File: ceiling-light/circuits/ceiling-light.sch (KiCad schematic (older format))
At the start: 33 parts, among them J1 Screw_Terminal_01x03, J2 Screw_Terminal_01x02, J3 Conn_02x04_Counter_Clockwise, Q2 IRF840, Q3 IRF840, Q4 KSP44, SW1 SW_Push, SW2 SW_Push, U1 LTV-817, U2 HLK-PM05, U3 AMS1117-3.3, U4 FL51xxMX, U5 TMP36xS, U6 ESP32-WROOM-32D

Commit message: removed old undimmable version
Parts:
- BR1: symbol ceiling-light-dimmable-rescue:DB107-BP-Diode_Bridge_slimc-ceiling-light-dimmable-rescue-ceiling-light-dimmable-rescue -> ceiling-light-rescue:DB107-BP-Diode_Bridge_slimc-ceiling-light-dimmable-rescue-ceiling-light-dimmable-rescue-ceiling-li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
- U4: symbol ceiling-light-dimmable-rescue:FL51xxMX-AC_Drivers_slimc-ceiling-light-dimmable-rescue-ceiling-light-dimmable-rescue -> ceiling-light-rescue:FL51xxMX-AC_Drivers_slimc-ceiling-light-dimmable-rescue-ceiling-light-dimmable-rescue-ceiling-ligh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
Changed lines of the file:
@@
 EESchema Schematic File Version 4
-LIBS:ceiling-light-dimmable-cache
+LIBS:ceiling-light-cache
 EELAYER 26 0
 EELAYER END
@@
 	6400 700  6400 4400
 $Comp
-L ceiling-light-dimmable-rescue:FL51xxMX-AC_Drivers_slimc-ceiling-light-dimmable-rescue-ceiling-light-dimmable-rescue U4
+L ceiling-light-rescue:FL51xxMX-AC_Drivers_slimc-ceiling-light-dimmable-rescue-ceiling-light-dimmable-rescue-ceiling-light-dimmable-rescue-ceiling-light-dimmable-rescue U4
 U 1 1 5D445EC1
 P 4600 1500
@@
 $EndComp
 $Comp
-L ceiling-light-dimmable-rescue:DB107-BP-Diode_Bridge_slimc-ceiling-light-dimmable-rescue-ceiling-light-dimmable-rescue BR1
+L ceiling-light-rescue:DB107-BP-Diode_Bridge_slimc-ceiling-light-dimmable-rescue-ceiling-light-dimmable-rescue-ceiling-light-dimmable-rescue-ceiling-light-dimmable-rescue BR1
 U 1 1 5D4584FE
 P 4400 3450

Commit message: new schematic layout
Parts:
- removed BR1: DB107-BP, Diode_THT_slimc:DB107-BP, symbol ceiling-light-rescue:DB107-BP-Diode_Bridge_slimc-ceiling-light-dimmable-rescue-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
- removed J3: Conn_02x04_Counter_Clockwise, Connector_PinSocket_2.54mm:PinSocket_2x04_P2.54mm_Vertical, symbol Connector_Generic:Conn_02x04_Counter_Clockwise
- removed R7: LDR03, OptoDevice:R_LDR_5.0x4.1mm_P3mm_Vertical, symbol Sensor_Optical:LDR03
- removed SW2: SW_Push, Button_Switch_THT:SW_Tactile_Straight_KSA0Axx1LFTR, symbol Switch:SW_Push
- removed U4: FL51xxMX, AC_Drivers_slimc:FL51xxMX, symbol ceiling-light-rescue:FL51xxMX-AC_Drivers_slimc-ceiling-light-dimmable-rescue-ce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
- added BR1: DB107-BP, DIP825W56P510L828H330Q4N, symbol Diode_Bridge_slimc:DB107-BP
- added J3: Conn_01x04, symbol Connector_Generic:Conn_01x04
- added R3: LDR03, OptoDevice:R_LDR_5.0x4.1mm_P3mm_Vertical, symbol Sensor_Optical:LDR03
- added R4: 6K8, Resistor_THT:R_Axial_DIN0207_L6.3mm_D2.5mm_P10.16mm_Horizontal, symbol Device:R
- added U4: FL51xxMX, symbol AC_Drivers_slimc:FL51xxMX
- C1, C4: value 100nF -> 100n
- C2: value 22nF -> 22n
- R6: value 6K8 -> 10K
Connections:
- net labels removed: +5V, ESP_EN, ESP_GPIO_00, ESP_GPIO_02, ESP_GPIO_04, ESP_GPIO_05, ESP_GPIO_12, ESP_GPIO_13, ESP_GPIO_14, ESP_GPIO_15, ESP_GPIO_16, ESP_GPIO_17, ESP_GPIO_18, ESP_GPIO_19, ESP_GPIO_21, ESP_GPIO_22, ESP_GPIO_23, ESP_GPIO_25, ESP_GPIO_26, ESP_GPIO_27, ESP_GPIO_33, ESP_GPIO_34, ESP_GPIO_35, ESP_RXD0, ESP_SENSOR_VN, ESP_SENSOR_VP, ESP_TXD0, L_M1, L_M2, L_OUT, N_MAIN
- wire segments 151 -> 157
- no-connect marks 22 -> 25
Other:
- note added: "AC LOAD OUTPUT"
- note added: "AC SENSE (ZERO CROSSING)"
- note added: "FTDI"
- note added: "LAMP SOCKET INPUT"
- note added: "LIGHT LEVEL SENSE"
- note added: "LOAD CONTROL (DIMMABLE)"
- note added: "MCU (ESP32)"
- note added: "PCB TEMP MONITOR"
- note added: "POWER SUPPLY"
- note removed: "3V3 DC CONVERTER"
- note removed: "5 : GND"
- note removed: "5V ACDC CONVERTER"
- note removed: "6 : GND"
- note removed: "7 : 5V PWR"
- note removed: "8 : 3V3 PWR"
- note removed: "ESP32-WROOM-32D MCU"
- note removed: "FTDI DTR -> ESP GPIO0 : 4"
- note removed: "FTDI RTS -> ESP EN : 3"
- note removed: "FTDI RXD -> ESP TXD : 1"
- note removed: "FTDI TXD -> ESP RXD : 2"
- note removed: "LIGHT SENSER"
- note removed: "MAINS INPUT"
- note removed: "MAINS OUTPUT"
- note removed: "MAINS POWER SENSE"
- note removed: "MAINS POWER SWITCHING"
- note removed: "PROGRAMMING HEADER"
- note removed: "TEMPERATURE SENSOR"
- moved on the sheet: C1, C2, C3, C4, D2, F1, J1, J2, Q2, Q3, Q4, R1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

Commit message: work on dimmable ceiling light
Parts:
- removed C1, C4: 100n, Capacitor_THT:CP_Radial_D5.0mm_P2.50mm, symbol Device:C_Small
- removed J3: Conn_01x04, symbol Connector_Generic:Conn_01x04
- removed U3: AMS1117-3.3, Package_TO_SOT_SMD:SOT-223-3_TabPin2, symbol Regulator_Linear:AMS1117-3.3
- added C1, C4: 0.1µ, Capacitor_THT:CP_Radial_D5.0mm_P2.50mm, symbol Device:CP
- added J3: Conn_01x06, symbol Connector_Generic:Conn_01x06
- added R7: 10K, Resistor_THT:R_Axial_DIN0207_L6.3mm_D2.5mm_P10.16mm_Horizontal, symbol Device:R
- added SW2: SW_Push, Button_Switch_THT:SW_Tactile_Straight_KSA0Axx1LFTR, symbol Switch:SW_Push
- BR1: value DB107-BP -> DB107; footprint DIP825W56P510L828H330Q4N -> (none)
- U2: value HLK-PM05 -> HLK-PM03
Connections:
- wire segments 157 -> 165
- no-connect marks 25 -> 24
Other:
- note added: "FTDI HEADER"
- note removed: "FTDI"
- moved on the sheet: C2, C3, C5, D1, D2, F1, J1, J2, Q2, Q3, Q4, R1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

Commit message: changed schematic layout
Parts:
- removed BR1: DB107, symbol Diode_Bridge_slimc:DB107-BP
- removed C1, C4, C5: 0.1µ, Capacitor_THT:CP_Radial_D5.0mm_P2.50mm, symbol Device:CP
- removed C2: 22n, Capacitor_THT:CP_Radial_D5.0mm_P2.50mm, symbol Device:C_Small
- removed C3: 4µ7, Capacitor_THT:CP_Radial_D5.0mm_P2.50mm, symbol Device:CP
- removed D1: WS2812B, LED_SMD:LED_WS2812B_PLCC4_5.0x5.0mm_P3.2mm, symbol LED:WS2812B
- removed D2: 1N4007, Diode_THT:D_DO-41_SOD81_P10.16mm_Horizontal, symbol Diode:1N4007
- removed F1: Fuse, Fuse_Holders_and_Fuses:Fuseholder5x20_horiz_open_lateral_Type-II, symbol Device:Fuse
- removed J1: Screw_Terminal_01x03, TerminalBlock:TerminalBlock_bornier-3_P5.08mm, symbol Connector:Screw_Terminal_01x03
- removed J2: Screw_Terminal_01x02, TerminalBlock:TerminalBlock_bornier-2_P5.08mm, symbol Connector:Screw_Terminal_01x02
- removed J3: Conn_01x06, symbol Connector_Generic:Conn_01x06
- removed Q2, Q3: IRF840, Package_TO_SOT_SMD:TO-263-3_TabPin2, symbol Transistor_FET:IRF740
- removed Q4: KSP44, Package_TO_SOT_THT:TO-92_Inline, symbol Transistor_BJT:2N2219
- removed R1: 390K, Resistor_THT:R_Axial_DIN0207_L6.3mm_D2.5mm_P10.16mm_Horizontal, symbol Device:R
- removed R10, R12, R13: 2M2, Resistor_THT:R_Axial_DIN0411_L9.9mm_D3.6mm_P12.70mm_Horizontal, symbol Device:R
- removed R11: 1K, Resistor_THT:R_Axial_DIN0207_L6.3mm_D2.5mm_P10.16mm_Horizontal, symbol Device:R
- removed R2, R6, R7: 10K, Resistor_THT:R_Axial_DIN0207_L6.3mm_D2.5mm_P10.16mm_Horizontal, symbol Device:R
- removed R3: LDR03, OptoDevice:R_LDR_5.0x4.1mm_P3mm_Vertical, symbol Sensor_Optical:LDR03
- removed R4: 6K8, Resistor_THT:R_Axial_DIN0207_L6.3mm_D2.5mm_P10.16mm_Horizontal, symbol Device:R
- removed R5: 330K, Resistor_THT:R_Axial_DIN0207_L6.3mm_D2.5mm_P10.16mm_Horizontal, symbol Device:R
- removed R9: 33K, Resistor_THT:R_Axial_DIN0207_L6.3mm_D2.5mm_P10.16mm_Horizontal, symbol Device:R
- removed SW1, SW2: SW_Push, Button_Switch_THT:SW_Tactile_Straight_KSA0Axx1LFTR, symbol Switch:SW_Push
- removed U1: LTV-817, Package_DIP:DIP-4_W7.62mm, symbol Isolator:LTV-817
- removed U2: HLK-PM03, Power_Supply:HLK-PM01, symbol Power_Supplies:HLK-PM05
- removed U4: FL51xxMX, symbol AC_Drivers_slimc:FL51xxMX
- removed U5: TMP36xS, Package_SO:SOIC-8_3.9x4.9mm_P1.27mm, symbol Sensor_Temperature:TMP36xS
- removed U6: ESP32-WROOM-32D, RF_Module:ESP32-WROOM-32, symbol RF_Module:ESP32-WROOM-32D
- added C? (x2): 0.1µ, Capacitor_THT:CP_Radial_D5.0mm_P2.50mm, symbol Device:CP
- added C?: 22n, Capacitor_THT:CP_Radial_D5.0mm_P2.50mm, symbol Device:C_Small
- added C? (x2): 0.1µ, symbol Device:CP_Small
- added C?: 22µ, symbol Device:CP_Small
- added C?: 4µ7, symbol Device:CP_Small
- added D?: WS2812B, LED_SMD:LED_WS2812B_PLCC4_5.0x5.0mm_P3.2mm, symbol LED:WS2812B
- added D?: 1N4007, Diode_THT:D_DO-41_SOD81_P10.16mm_Horizontal, symbol Diode:1N4007
- added D?: D_Bridge_+-AA, symbol Device:D_Bridge_+-AA
- added F? (x2): Fuse, Fuse_Holders_and_Fuses:Fuseholder5x20_horiz_open_lateral_Type-II, symbol Device:Fuse
- added J?: Screw_Terminal_01x03, TerminalBlock:TerminalBlock_bornier-3_P5.08mm, symbol Connector:Screw_Terminal_01x03
- added J?: Screw_Terminal_01x02, TerminalBlock:TerminalBlock_bornier-2_P5.08mm, symbol Connector:Screw_Terminal_01x02
- added J?: Conn_01x06, symbol Connector_Generic:Conn_01x06
- added PS?: IRM-02-5, Converter_ACDC:Converter_ACDC_MeanWell_IRM-02-xx_THT, symbol Converter_ACDC:IRM-02-5
- added Q? (x2): IRF840, Package_TO_SOT_SMD:TO-263-3_TabPin2, symbol Transistor_FET:IRF740
- added Q?: KSP44, Package_TO_SOT_THT:TO-92_Inline, symbol Transistor_BJT:2N2219
- added R?: 10K, Resistor_THT:R_Axial_DIN0207_L6.3mm_D2.5mm_P10.16mm_Horizontal, symbol Device:R
- added R?: 390K, Resistor_THT:R_Axial_DIN0207_L6.3mm_D2.5mm_P10.16mm_Horizontal, symbol Device:R
- added R? (x3): 2M2, symbol Device:R_Small
- added R?: 1K, symbol Device:R_Small
- added R?: 330K, symbol Device:R_Small
- added R?: 33K, symbol Device:R_Small
- added R? (x2): 10K, symbol Device:R_Small
- added SW? (x2): SW_Push, Button_Switch_THT:SW_Tactile_Straight_KSA0Axx1LFTR, symbol Switch:SW_Push
- added U?: ESP32-WROOM-32D, RF_Module:ESP32-WROOM-32, symbol RF_Module:ESP32-WROOM-32D
- added U?: AMS1117-3.3, Package_TO_SOT_SMD:SOT-223-3_TabPin2, symbol Regulator_Linear:AMS1117-3.3
- added U?: TMP36xS, Package_SO:SOIC-8_3.9x4.9mm_P1.27mm, symbol Sensor_Temperature:TMP36xS
- added U?: FL51xxMX, symbol AC_Drivers_slimc:FL51xxMX
- added U?: LTV-817, Package_DIP:DIP-4_W7.62mm, symbol Isolator:LTV-817
- added U?: DAC081C081CIMK, Package_TO_SOT_SMD:SOT-23-6, symbol Analog_DAC:DAC081C081CIMK
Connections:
- net labels added: +5V, DIMCN_V, ESP32_BOOT, ESP32_RST, ESP32_RXD, ESP32_SCL, ESP32_SDA, ESP32_TXD, MAINS_L_IN, MAINS_L_IN_SW, MAINS_L_OUT, MAINS_N, PCB_TEMP_SENSE, STATUS_LED, SW_SENSE
- wire segments 165 -> 139
- no-connect marks 24 -> 6
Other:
- note added: "FTDI PROG HEADER"
- note added: "MAINS INTERFACE"
- note added: "MICROCONTROLLER"
- note added: "PCB TEMP SENSOR"
- note added: "POWER SUPPLIES"
- note added: "PUSH BUTTONS"
- note added: "STATUS LED"
- note removed: "AC LOAD OUTPUT"
- note removed: "CONSTANT"
- note removed: "FTDI HEADER"
- note removed: "LAMP SOCKET INPUT"
- note removed: "LIGHT LEVEL SENSE"
- note removed: "LIVE LOAD"
- note removed: "MCU (ESP32)"
- note removed: "NEUTRAL"
- note removed: "PCB TEMP MONITOR"
- note removed: "POWER SUPPLY"
- note removed: "RGB STATUS LED"
- note removed: "SWITCH"

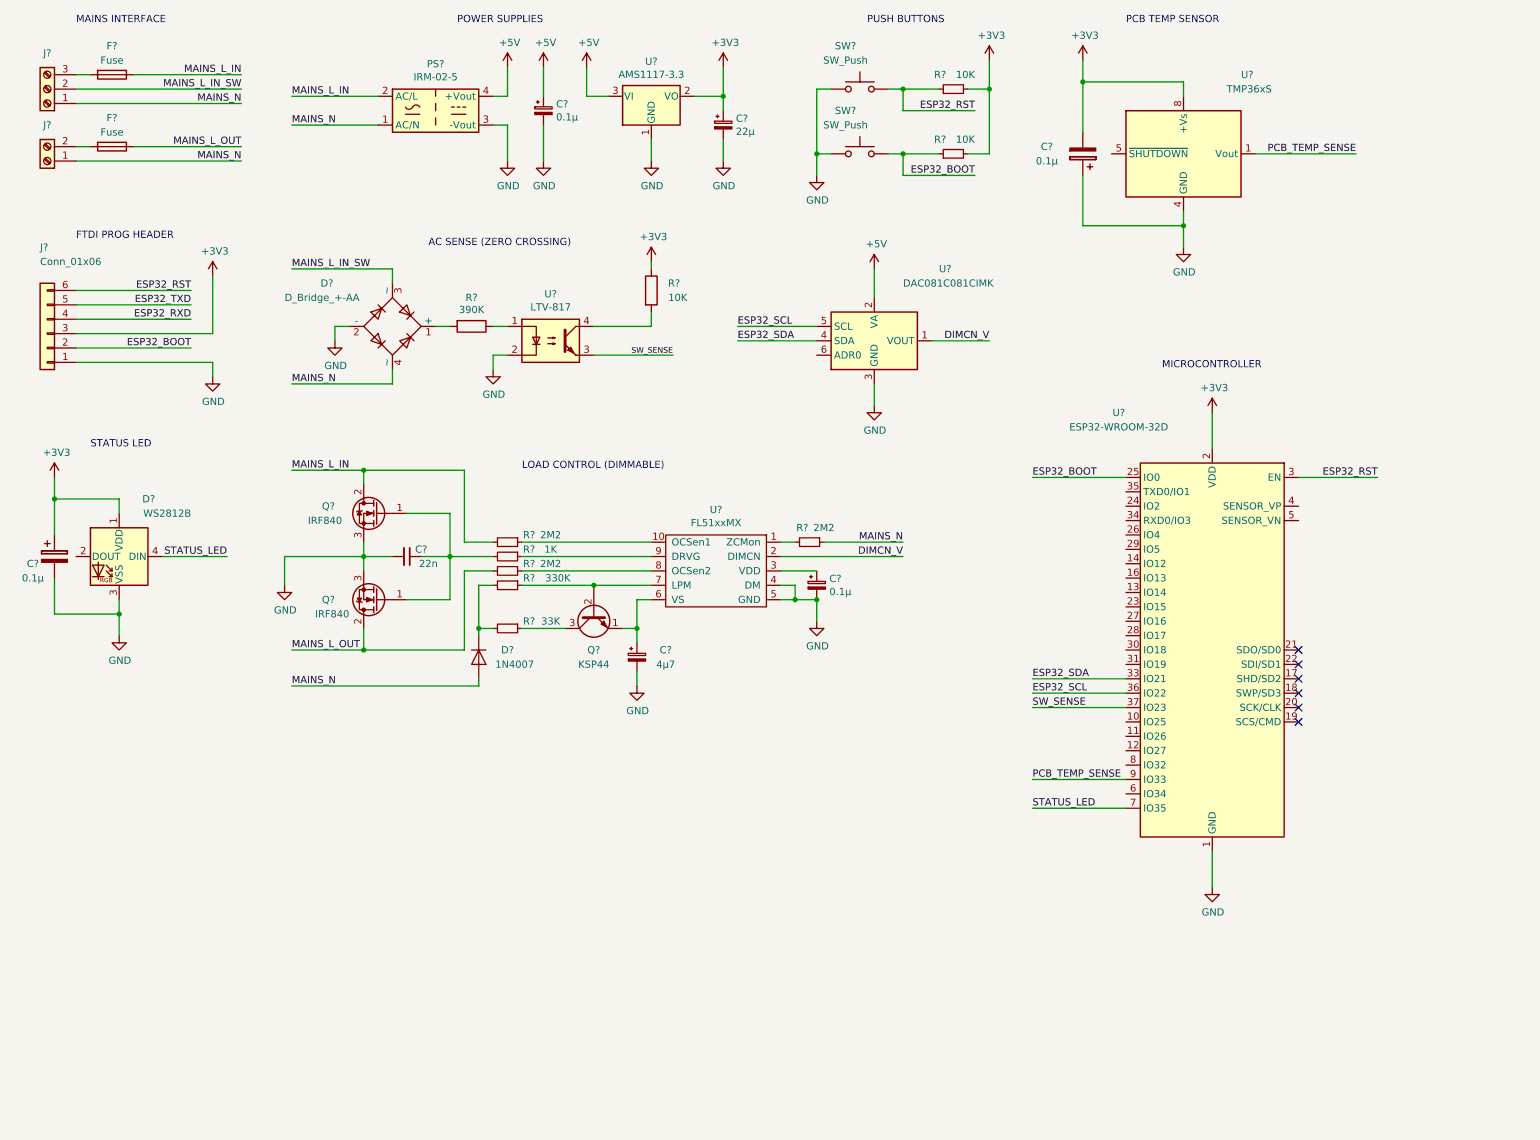
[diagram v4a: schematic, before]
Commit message: improving schematic
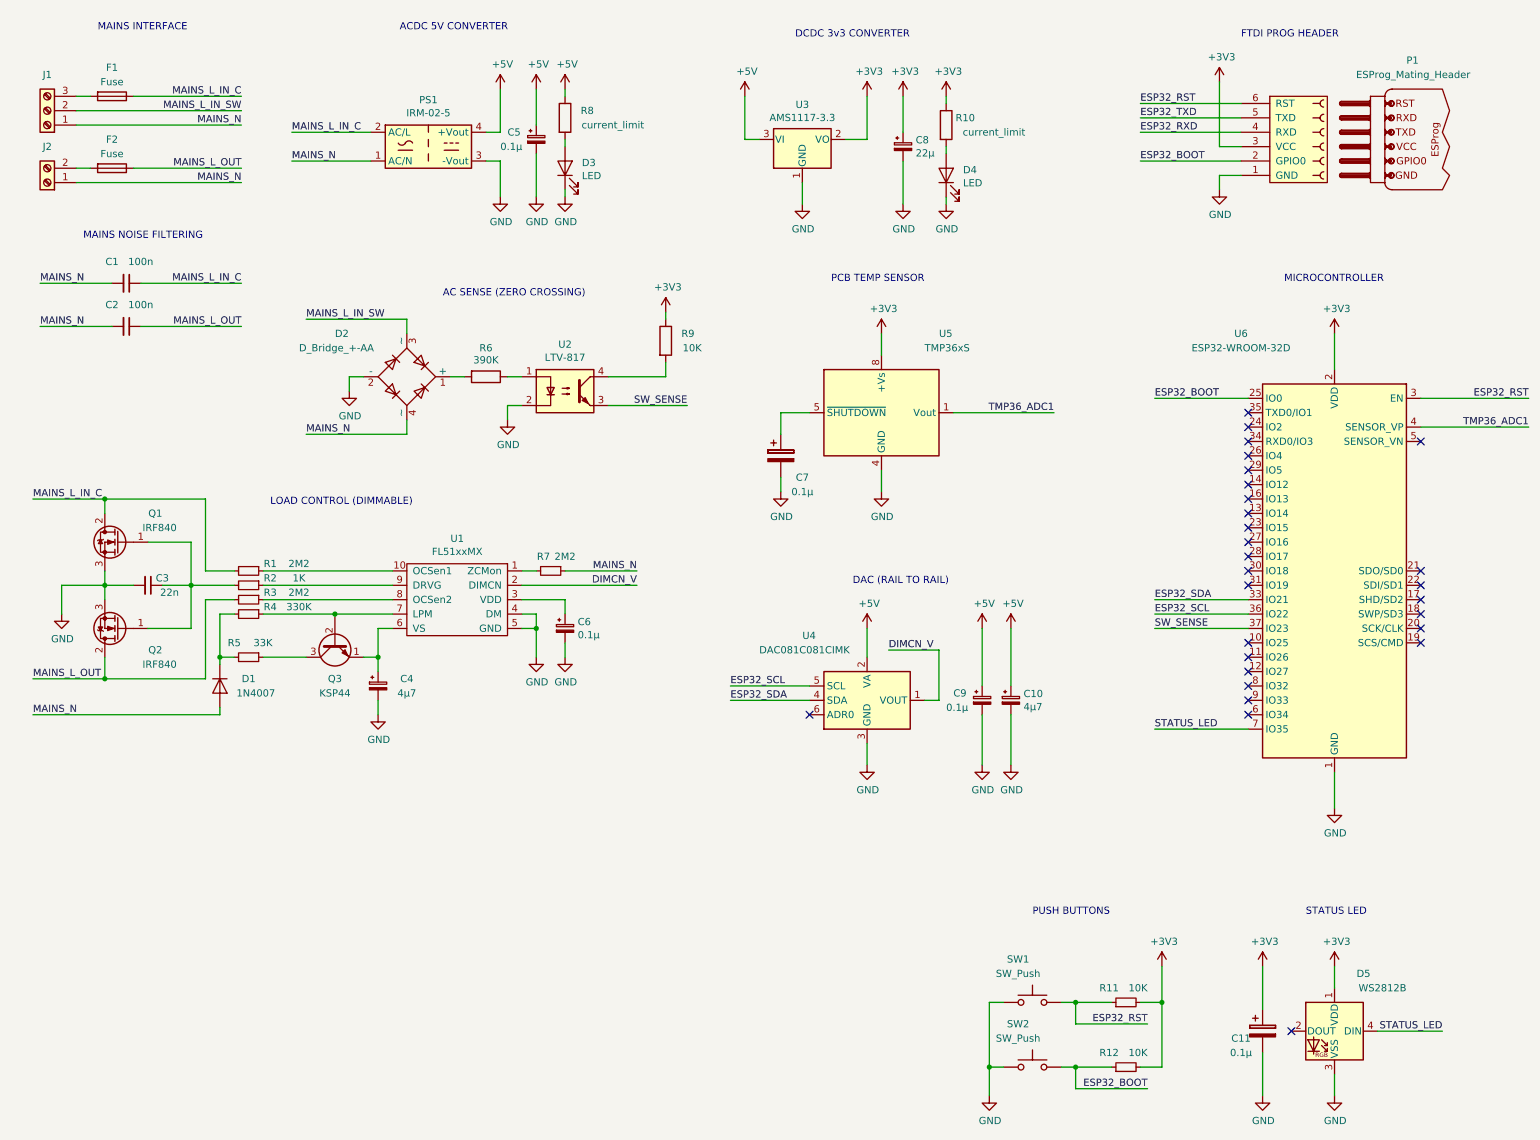
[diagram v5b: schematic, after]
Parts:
- removed J?: Conn_01x06, symbol Connector_Generic:Conn_01x06
- added C1, C2: 100n, Capacitor_THT:CP_Radial_D5.0mm_P2.50mm, symbol Device:C_Small
- added C10: 4µ7, symbol Device:CP_Small
- added C9: 0.1µ, symbol Device:CP_Small
- added D3, D4: LED, symbol Device:LED
- added P1: ESProg_Mating_Header, footprints:ESProg_PinSocket_1x06_P2.54mm_Vertical, symbol ESProg:ESProg_Mating_Header
- added R10, R8: current_limit, Resistor_THT:R_Axial_DIN0207_L6.3mm_D2.5mm_P10.16mm_Horizontal, symbol Device:R
- gave numbers to parts that had none: 36
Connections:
- net +3V3: now also P1.3 (VCC), R10.1; no longer C7.2
- net +5V: now also C10.1, C9.1, R8.1
- net ESP32_BOOT: now also P1.2 (GPIO0)
- net ESP32_RST: now also P1.6 (RST)
- net ESP32_RXD: now also P1.4 (RXD)
- net ESP32_TXD: now also P1.5 (TXD)
- net GND: now also C7.2, C10.2, C9.2, D3.1 (K), D4.1 (K), P1.1 (GND); no longer C7.1
- net MAINS_L_OUT: now also C2.1
- net MAINS_N: now also C1.2, C2.2
- net TMP36_ADC1: now reaches U6.4 (SENSOR_VP)
- net TMP36_ADC1: now also U5.1 (Vout)
- net at U5.5 (~SHUTDOWN): now also C7.1
- net MAINS_L_IN renamed MAINS_L_IN_C
- net MAINS_L_IN_C: now also C1.1
- net PCB_TEMP_SENSE: no longer names the net of U6.9 (IO33)
- net PCB_TEMP_SENSE: no longer U5.1 (Vout)
- new net: D3.2 (A), R8.2
- new net: D4.2 (A), R10.2
- no-connect marks 6 -> 28
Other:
- note added: "ACDC 5V CONVERTER"
- note added: "DAC (RAIL TO RAIL)"
- note added: "DCDC 3v3 CONVERTER"
- note added: "MAINS NOISE FILTERING"
- note removed: "POWER SUPPLIES"
- moved on the sheet: C11, C3, C4, C5, C6, C7, C8, D1, D2, D5, F1, F2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
